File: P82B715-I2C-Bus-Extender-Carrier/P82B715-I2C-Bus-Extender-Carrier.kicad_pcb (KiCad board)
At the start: 2 copper layers, 11 parts, among them IC1 P82B715TD,112, J1 Screw_Terminal_01x03, J2 Screw_Terminal_01x04, Q1 BD140

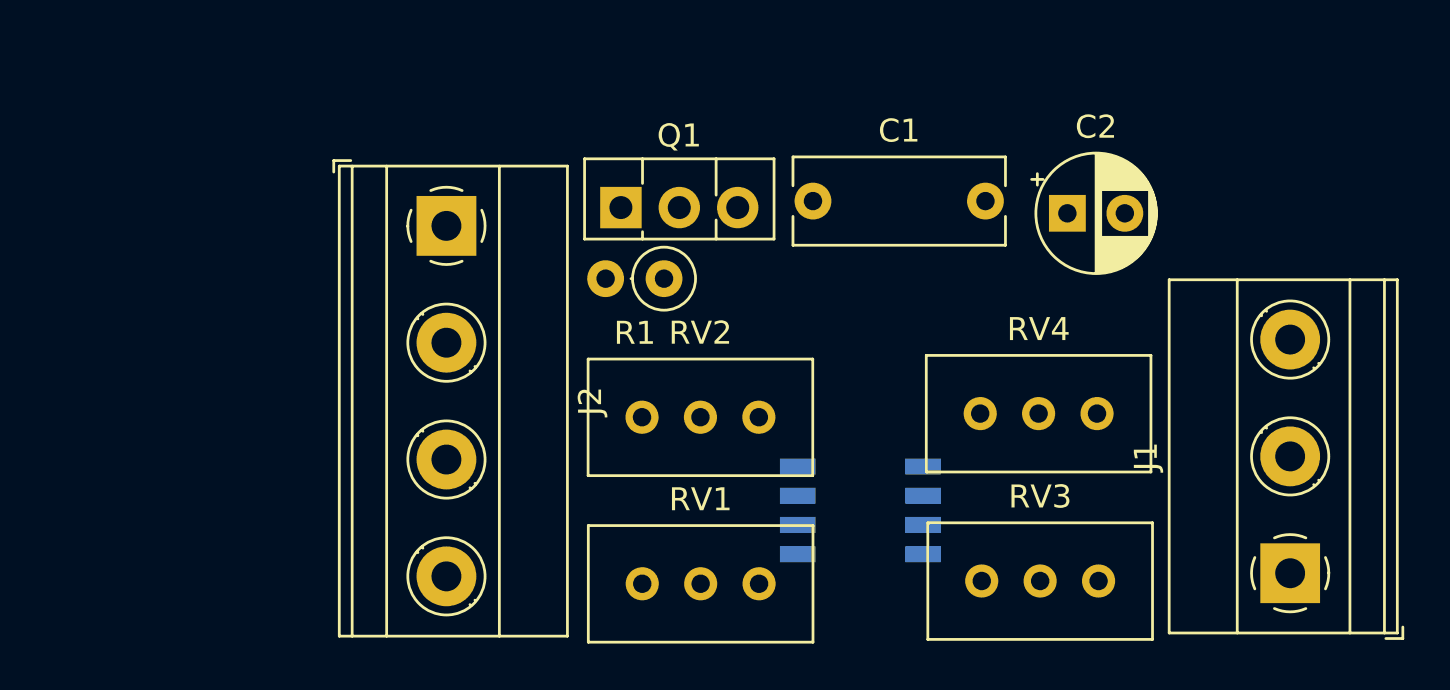
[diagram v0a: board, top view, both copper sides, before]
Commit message: routed and laid out. Fab Files included.
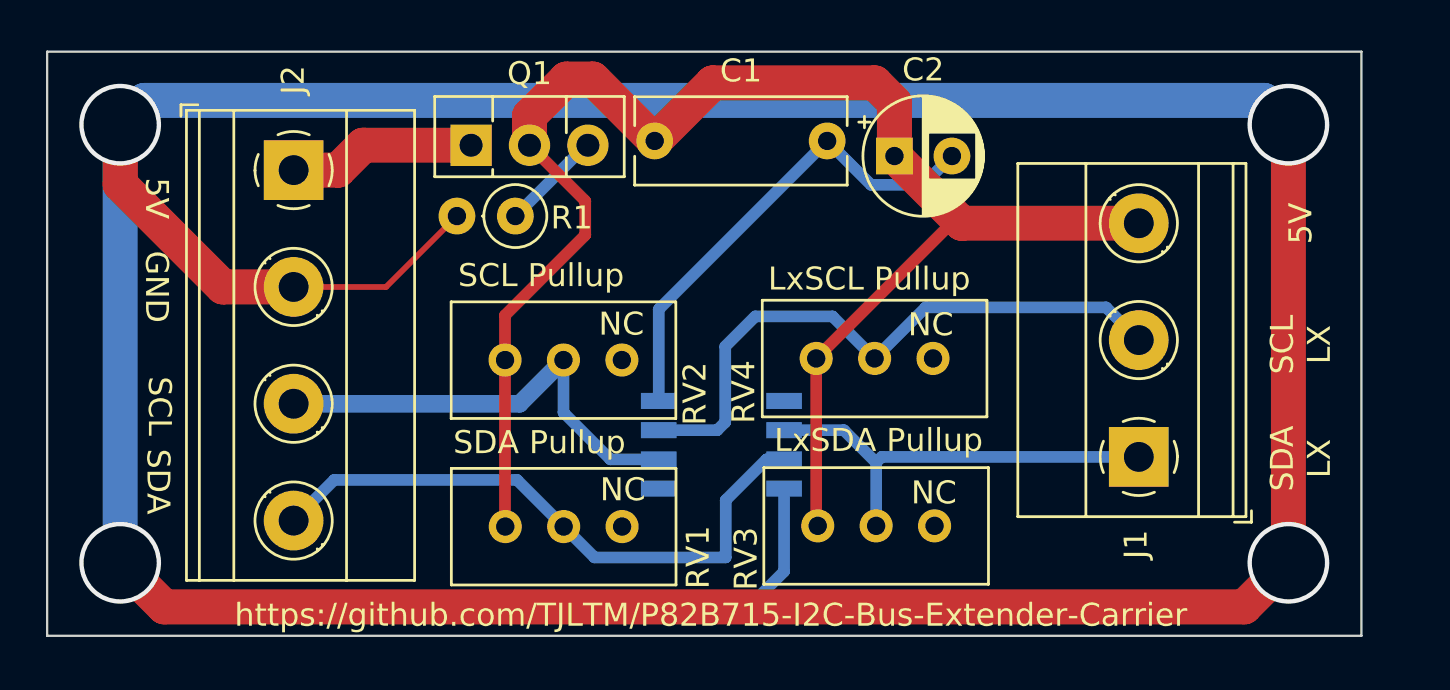
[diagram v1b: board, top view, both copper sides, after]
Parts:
- moved J1 8.30 mm to (149.1, 93.8)
- moved C2 7.92 mm to (138.4, 80.7)
- moved RV3 7.52 mm to (140.2, 96.8)
- moved RV4 7.52 mm to (140.1, 89.5)
- moved C1 7.36 mm to (128.0, 80.1)
- moved J2 7.07 mm to (112.3, 81.3)
- moved Q1 7.06 mm to (120.0, 80.3)
- moved R1 7.02 mm to (122.0, 83.3)
- moved IC1 6.68 mm to (130.9, 93.3)
- moved RV2 6.45 mm to (126.6, 89.6)
- moved RV1 6.45 mm to (126.6, 96.9)
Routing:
- net GND: track 0.00 -> 197.0 mm, vias 0 -> 4
- net +5V: track 0.00 -> 69.6 mm
- net BufferedSCL: track 0.00 -> 27.1 mm
- net SDA: track 0.00 -> 26.7 mm
- net Net-(C1-Pad2): track 0.00 -> 21.1 mm
- net SCL: track 0.00 -> 19.8 mm
- net BufferedSDA: track 0.00 -> 18.9 mm
- net Net-(J2-Pad1): track 0.00 -> 8.17 mm
- net Net-(Q1-Pad3): track 0.00 -> 4.43 mm
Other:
- board outline added: 57.2 x 25.4 mm
- board text added: "5V"
- board text added: "GND"
- board text added: "LxSCL Pullup"
- board text added: "LxSDA Pullup"
- board text added: "NC"
- board text added: "SCL"
- board text added: "SCL LX"
- board text added: "SCL Pullup"
- board text added: "SDA"
- board text added: "SDA LX"
- board text added: "SDA Pullup"
- board text added: "https://github.com/TJLTM/P82B715-I2C-Bus-Extender-Carrier"
